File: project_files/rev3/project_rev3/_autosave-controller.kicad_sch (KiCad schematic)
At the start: 26 parts, among them J8 USB_C_Receptacle_USB2.0_16P, SW1 JS102011SAQN, SW2 PTS810 SJM 250 SMTR LFS, SW3 PTS810 SJM 250 SMTR LFS, U5 ESP32-S3-WROOM-1-N16R8, U6 AZ1117CH-3.3

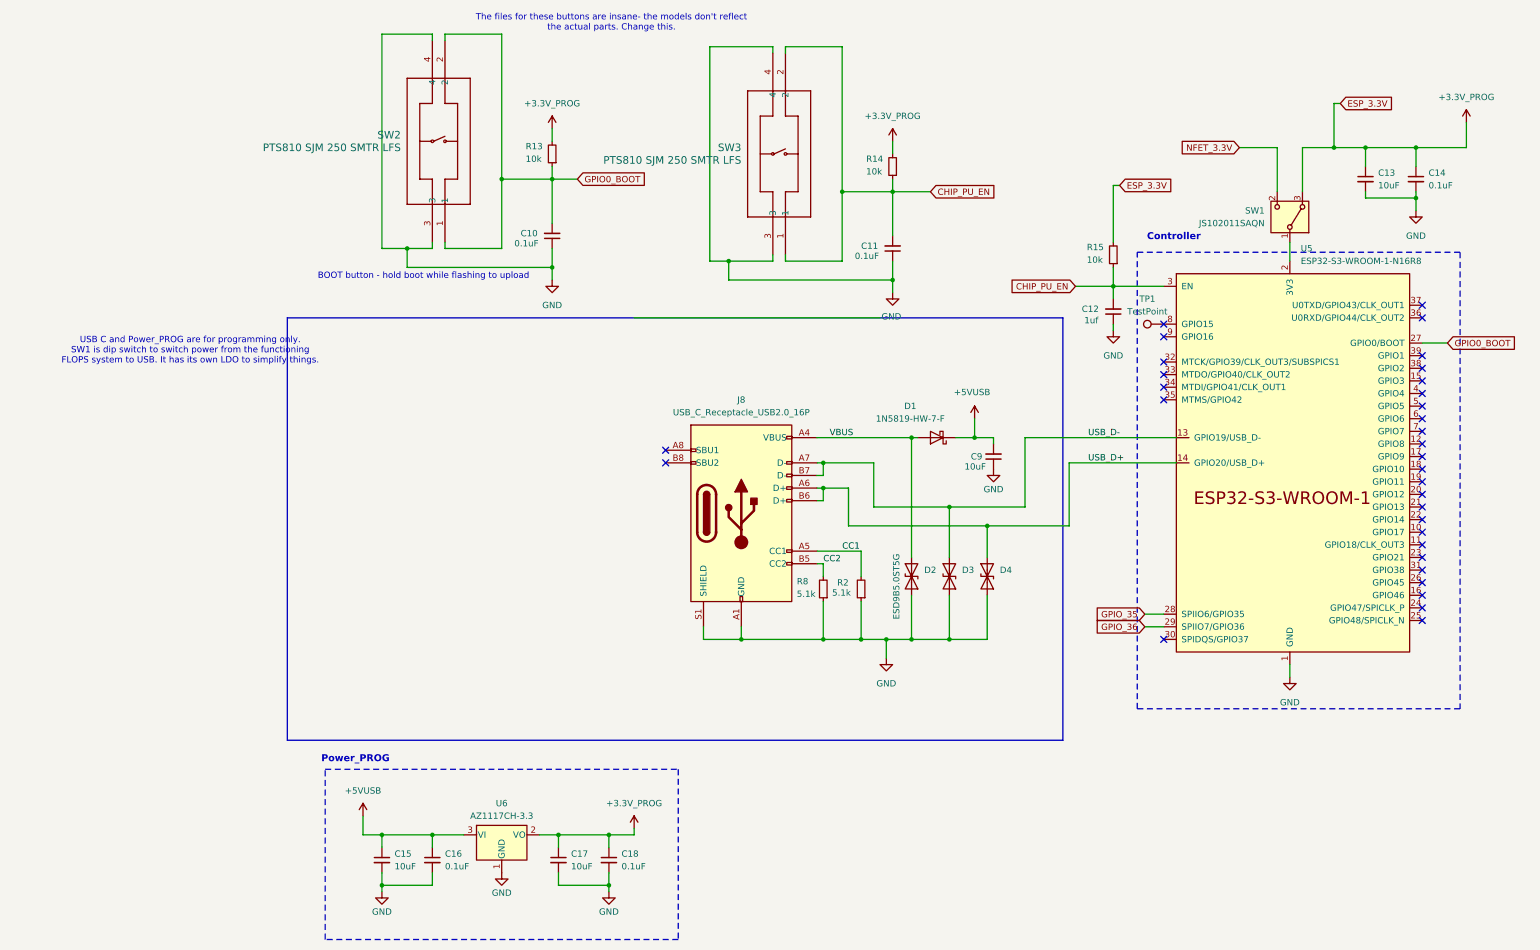
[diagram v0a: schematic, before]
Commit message: making a commit, didn't mean to do it on main but here we are
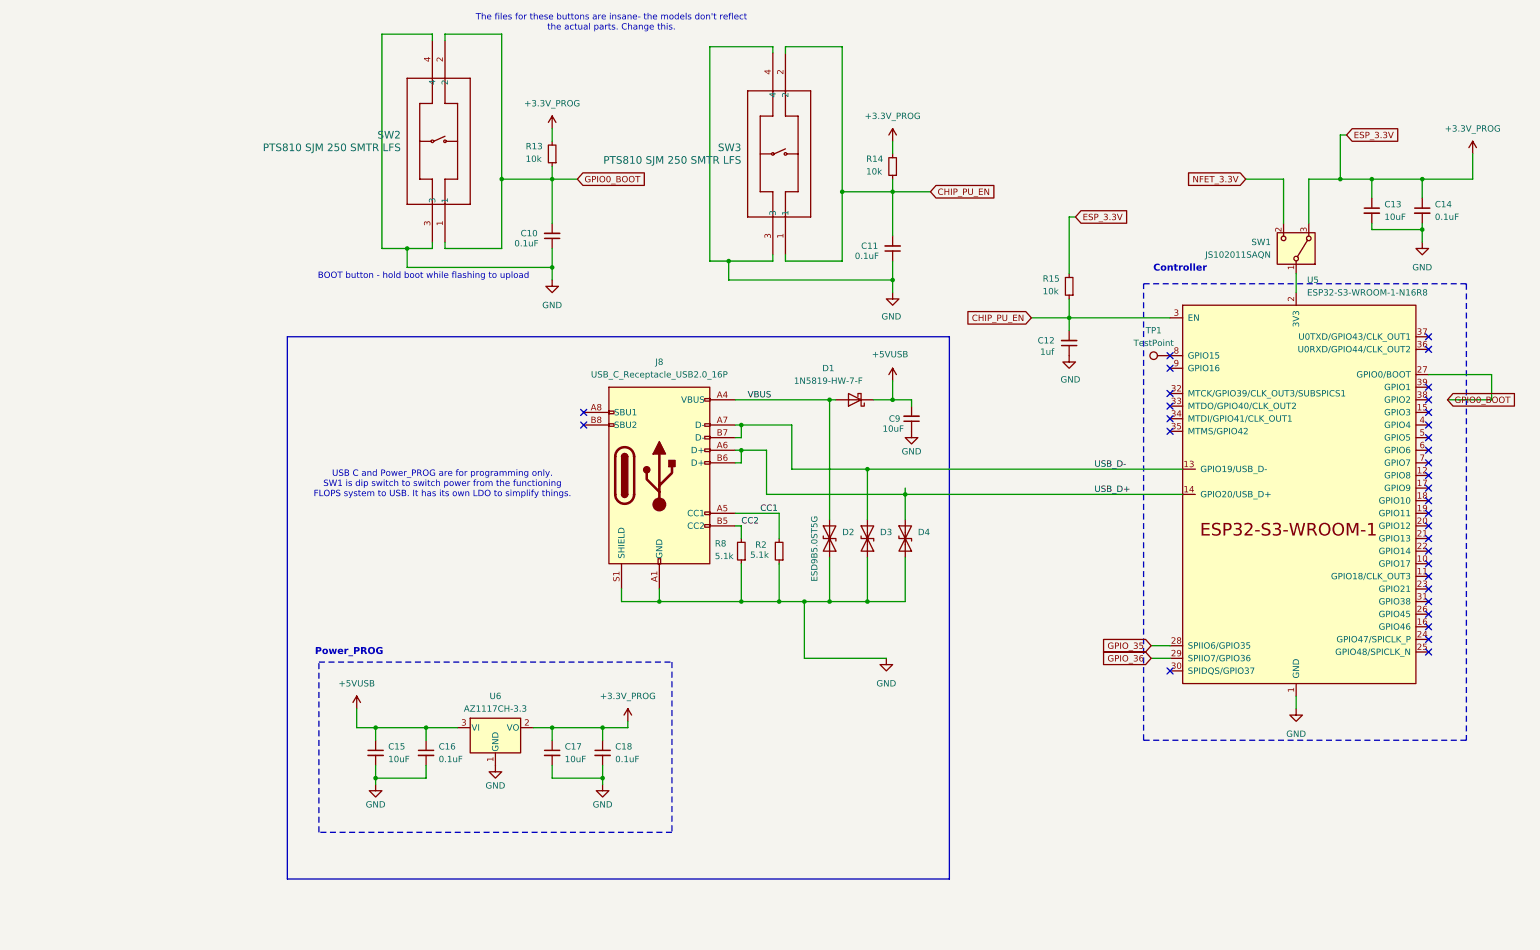
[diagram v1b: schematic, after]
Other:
- moved on the sheet: C12, C13, C14, C15, C16, C17, C18, C9, D1, D2, D3, D4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
